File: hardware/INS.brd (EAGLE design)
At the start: 47 x 40.5 mm, 47 parts, among them IC1 BN055, IC3 BME280, J1 MICRO_USB_B_HIROSE_ZX62-B-5PA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, U1 NEO-M9N-00B, U2 STM32L433CCT6

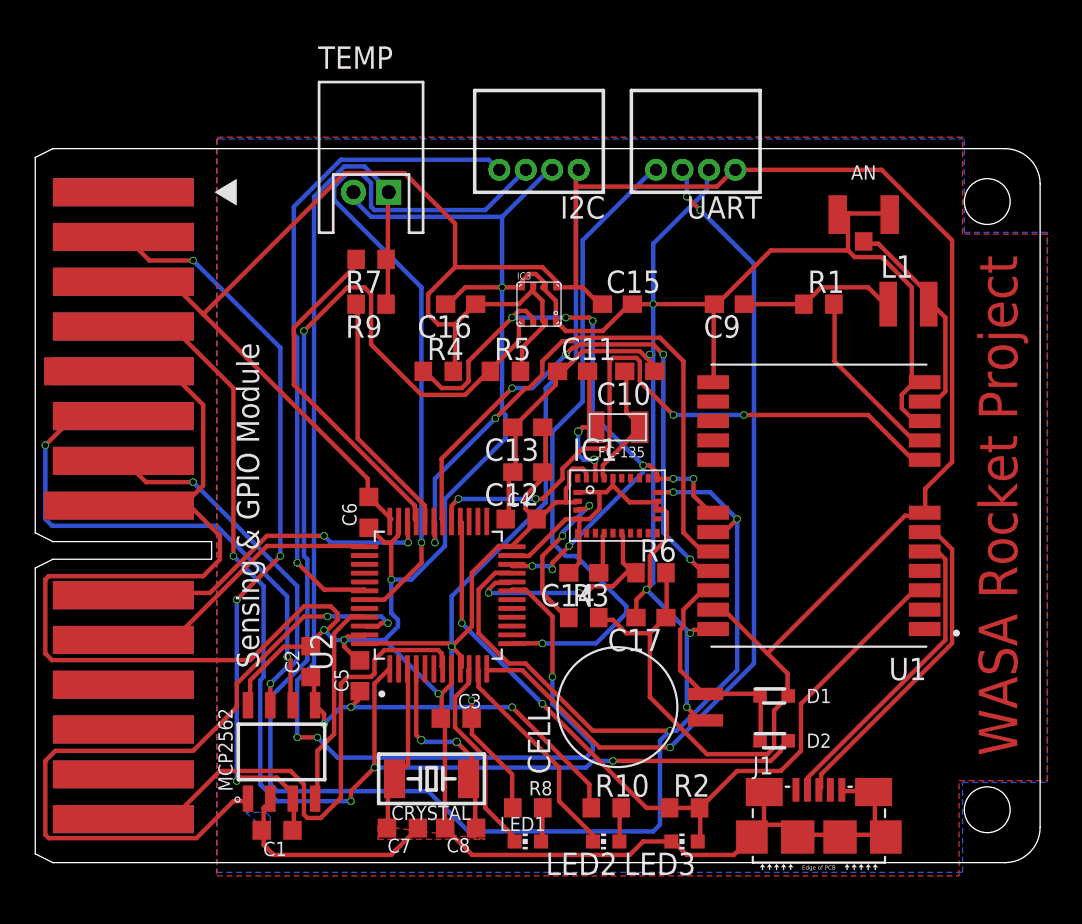
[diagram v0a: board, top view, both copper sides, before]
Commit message: 大変お待たせしました。BatteryPowerV2とINSの改良版です。確認お願いします。
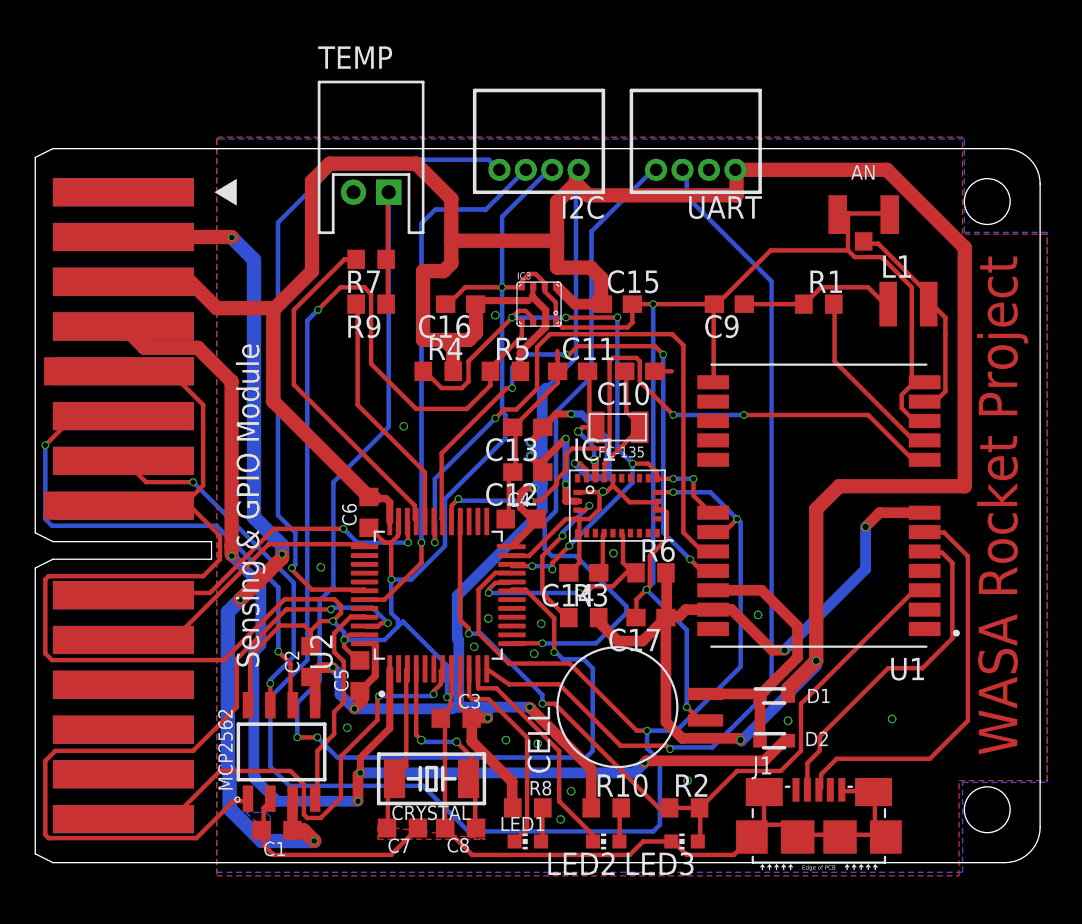
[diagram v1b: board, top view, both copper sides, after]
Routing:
- net VDD: track 251.6 -> 298.7 mm, vias 5 -> 15
- net GND: track 307.9 -> 288.9 mm, vias 10 -> 26
- net I2C1_SDA: track 41.3 -> 30.5 mm
- net VCC: track 42.9 -> 50.7 mm
- net USB_D+: track 18.7 -> 22.9 mm
- net N$11: track 13.4 -> 16.8 mm
- net N$4: track 30.4 -> 27.5 mm, vias 0 -> 2
- net TEMP: track 72.2 -> 69.3 mm
- net UART_TRX: track 48.7 -> 50.9 mm, vias 3 -> 1
- net VBAT: track 69.1 -> 71.1 mm
- net I2C2_SCL: track 114.2 -> 115.9 mm
- net GPS_RTX: track 35.1 -> 36.7 mm
- net USB_D-: track 17.7 -> 19.3 mm
- net I2C1_SCL: track 37.8 -> 39.1 mm
- net CAN_TX: track 41.9 -> 43.1 mm
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
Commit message: 微調整
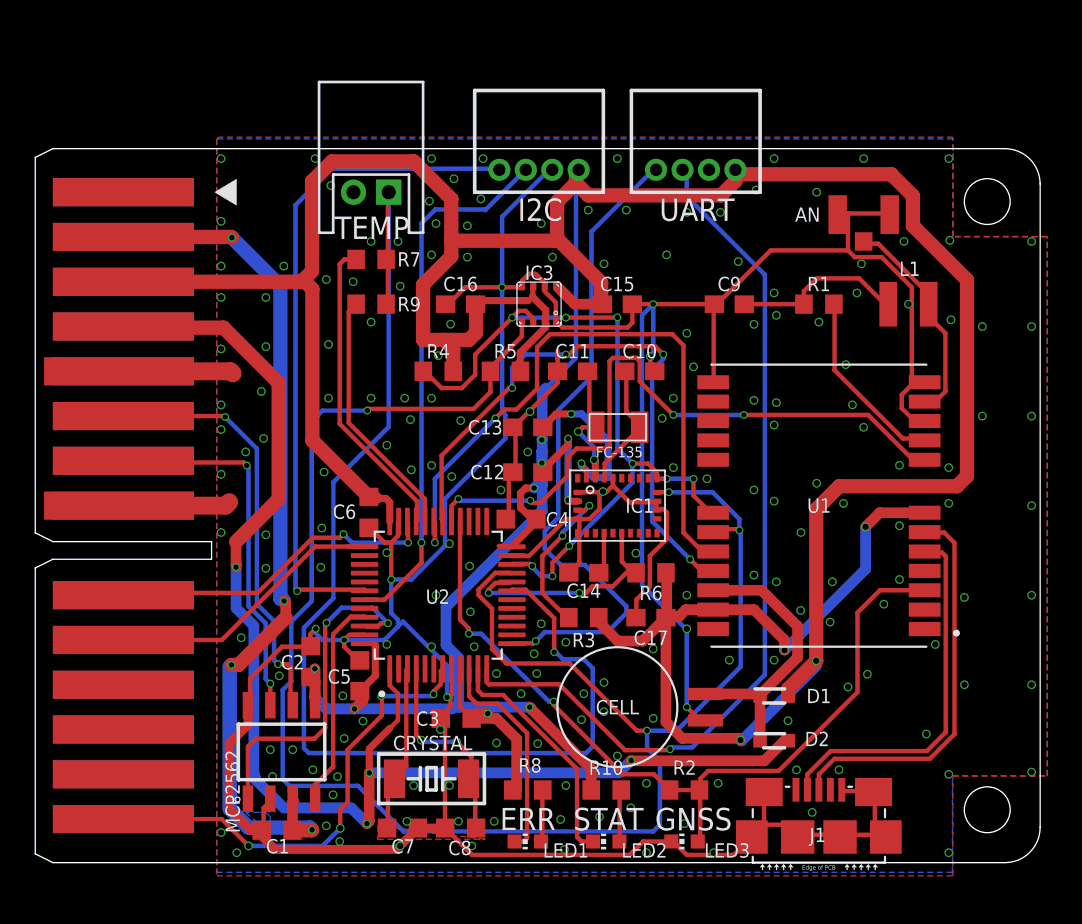
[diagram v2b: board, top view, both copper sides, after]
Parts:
- moved R10 1.02 mm to (32.4, -16.1)
- moved R2 1.02 mm to (36.8, -16.1)
- moved R8 1.02 mm to (27.9, -16.1)
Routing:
- net GND: track 288.9 -> 254.5 mm, vias 26 -> 198
- net CAN_TX: track 43.1 -> 19.4 mm
- net I2C2_SCL: track 115.9 -> 104.1 mm
- net CANL1: track 31.2 -> 24.1 mm
- net VDD: track 298.7 -> 292.8 mm
- net VBAT: track 71.1 -> 75.7 mm
- net TEMP_HIGH: track 19.6 -> 17.5 mm
- net USB_D-: track 19.3 -> 21.0 mm
- net 1PPS: track 45.5 -> 47.0 mm
- net CANH1: track 20.0 -> 21.2 mm
- net N$74: track 2.00 -> 3.02 mm
- net N$12: track 2.01 -> 3.02 mm
- net N$4: track 27.5 -> 26.5 mm, vias 2 -> 4
- net N$7: track 8.95 -> 9.80 mm
- net I2C1_SCL: track 39.1 -> 38.3 mm
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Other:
- board text added: "ERR"
- board text added: "GNSS"
- board text added: "INS Module"
- board text added: "STAT"
- board text added: "WASA Rocket 2023"
- board text removed: "Sensing & GPIO Module"
- board text removed: "WASA Rocket Project"
